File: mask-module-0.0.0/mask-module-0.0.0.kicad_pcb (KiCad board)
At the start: 2 copper layers, 17.8 x 33 mm, 27 parts, among them J1 Conn_01x02, J2 USB_C_Receptacle_USB2.0, J3 Conn_ARM_JTAG_SWD_10, J4 Conn_01x02, J5 Conn_01x13, J6 Conn_01x13, U1 BQ24075RGT, U3 MCP1703Ax-330xxTT, U4 BMD-380, Y1 FC-135 32.768KA-A5

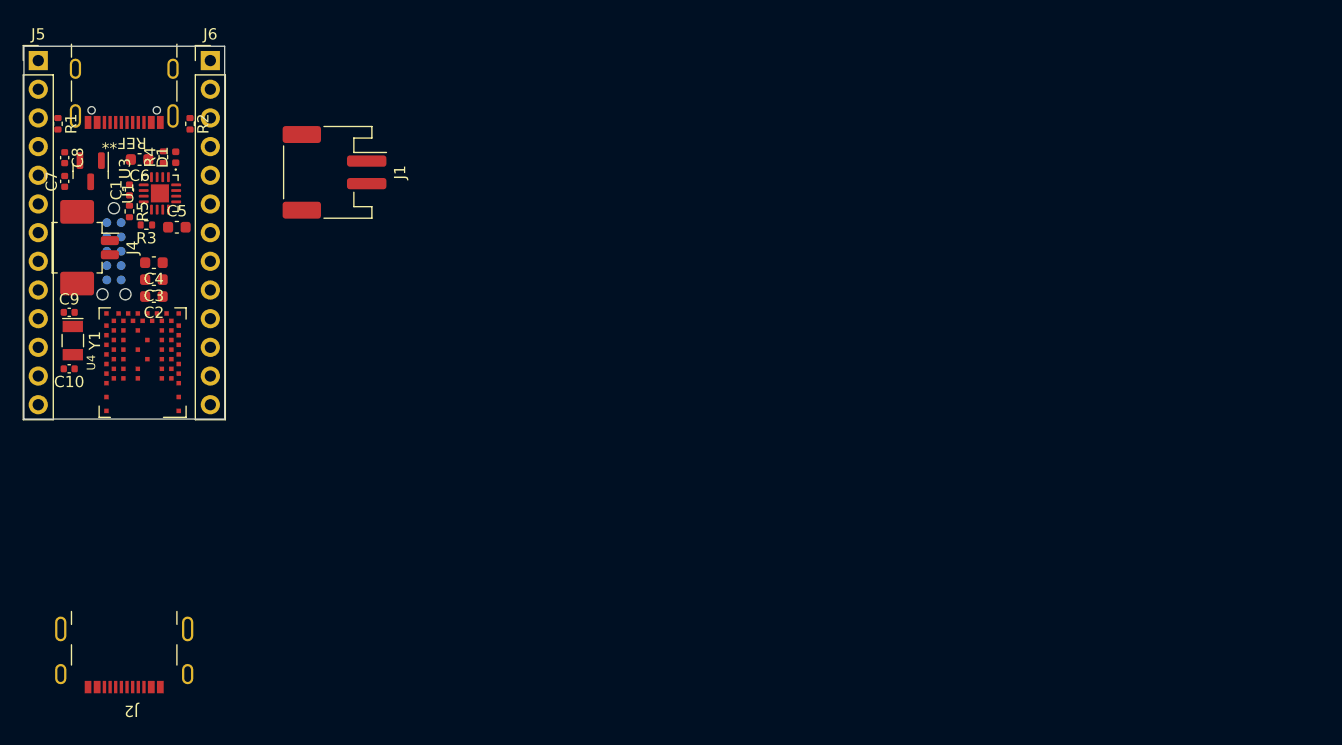
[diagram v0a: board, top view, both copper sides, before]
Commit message: module-0.0.0: finish pcb
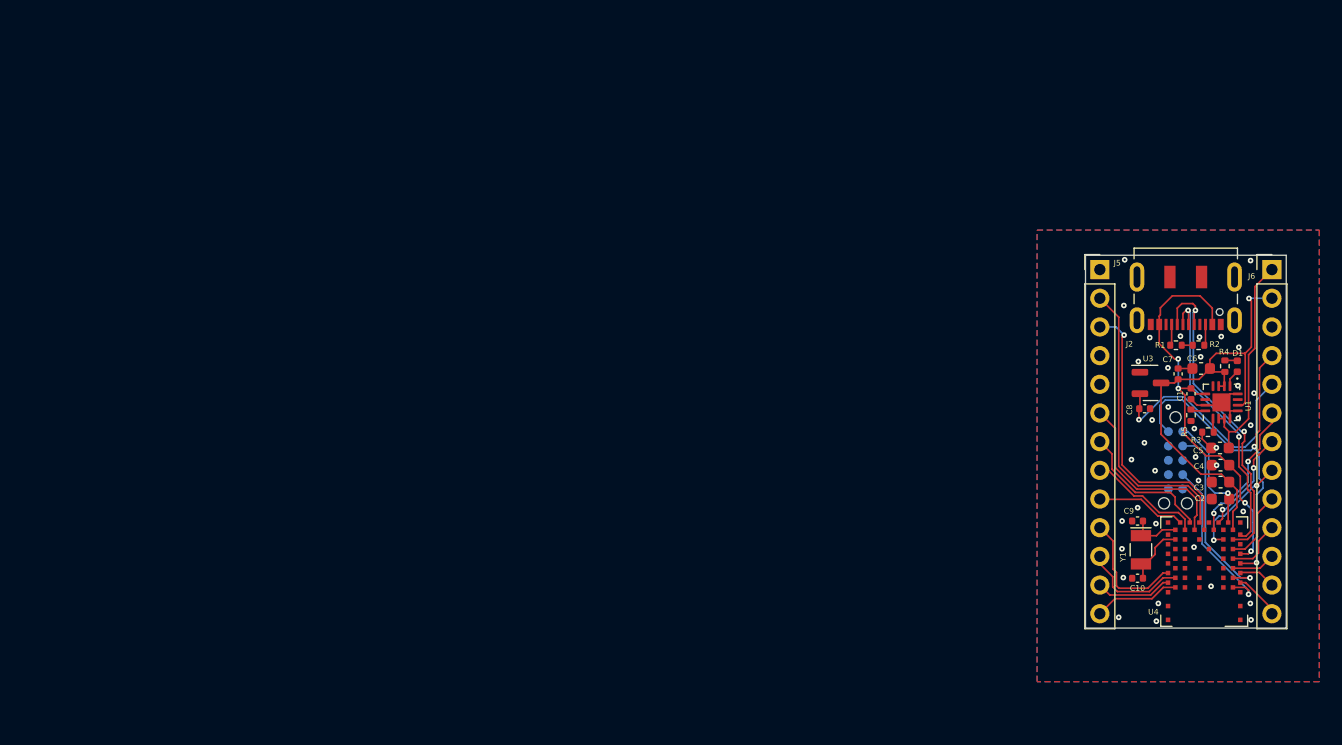
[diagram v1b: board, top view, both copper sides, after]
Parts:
- removed J1: Conn_01x02, Connector_JST:JST_PH_S2B-PH-SM4-TB_1x02-1MP_P2.00mm_Horizontal
- removed J4: Conn_01x02, Connector_Molex:Molex_PicoBlade_53261-0271_1x02-1MP_P1.25mm_Horizontal
- removed REF**: USB_C_Receptacle_GCT_USB4105-xx-A_16P_TopMnt_Horizontal, Connector_USB:USB_C_Receptacle_GCT_USB4105-xx-A_16P_TopMnt_Horizontal
- J2: footprint mask:USB_C_Receptacle_GCT_USB4520-xx-x-A_16P_Horizontal -> Connector_USB:USB_C_Receptacle_JAE_DX07S016JA1R1500
- moved R1 100.9 mm to (136.3, 88.7), turned to 0 degrees
- moved C7 100.1 mm to (136.5, 91.3)
- moved J2 99.3 mm to (137.2, 83.8)
- moved C8 98.2 mm to (133.6, 94.3), turned to 0 degrees
- moved C10 96.4 mm to (132.9, 109.4)
- moved C9 96.4 mm to (132.9, 104.3)
- moved Y1 96.4 mm to (133.2, 106.8)
- moved C2 96.2 mm to (140.3, 102.3)
- moved C3 96.2 mm to (140.3, 100.8)
- moved C4 96.2 mm to (140.3, 99.3)
- moved C6 95.8 mm to (138.6, 90.8)
- moved J5 95.8 mm to (129.6, 82.0)
- moved R4 95.8 mm to (140.7, 90.6)
- moved D1 95.8 mm to (141.8, 90.6)
- moved J3 95.8 mm to (136.3, 98.9)
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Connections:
- J5 pad 10: P1.00 -> P1.10
- J5 pad 11: P0.11 -> P1.06
- J5 pad 12: P1.04 -> P0.10
- J5 pad 13: P1.06 -> P0.09
- J5 pad 6: P0.17 -> P0.05
- J5 pad 7: P0.20 -> P0.27
- J5 pad 8: P0.22 -> P0.26
- J5 pad 9: P0.24 -> P0.04
- J6 pad 10: P1.13 -> P0.17
- J6 pad 11: P1.11 -> P0.21
- J6 pad 12: P0.10 -> P0.19
- J6 pad 13: P0.09 -> P0.22
- J6 pad 6: P0.31 -> P0.07
- J6 pad 7: P0.29 -> P0.12
- J6 pad 8: P0.02 -> P0.15
- J6 pad 9: P1.15 -> P0.14
- U4 pad 10: unconnected-(U4-P0.21-Pad10) -> P0.21
- U4 pad 16: unconnected-(U4-P0.14-Pad16) -> P0.14
- U4 pad 20: unconnected-(U4-P0.15-Pad20) -> P0.15
- U4 pad 26: unconnected-(U4-P0.12/TRACEDATA[1]-Pad26) -> P0.12
- U4 pad 27: unconnected-(U4-P0.07/TRACECLK-Pad27) -> P0.07
- U4 pad 31: unconnected-(U4-P0.05/AIN3-Pad31) -> P0.05
- U4 pad 32: unconnected-(U4-P0.27-Pad32) -> P0.27
- U4 pad 33: unconnected-(U4-P0.26-Pad33) -> P0.26
- U4 pad 34: unconnected-(U4-P0.04/AIN2-Pad34) -> P0.04
- U4 pad 49: unconnected-(U4-P1.10-Pad49) -> P1.10
- U4 pad 8: unconnected-(U4-P0.25-Pad8) -> P0.25
- U4 pad 9: unconnected-(U4-P0.19-Pad9) -> P0.19
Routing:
- net +5V: track 0.00 -> 41.6 mm, vias 0 -> 1
- net VBUS: track 0.00 -> 36.6 mm, vias 0 -> 4
- net RESET: track 0.00 -> 34.1 mm, vias 0 -> 2
- net D-: track 0.00 -> 29.4 mm, vias 0 -> 2
- net P0.06_TXD: track 0.00 -> 26.2 mm
- net D+: track 0.00 -> 25.8 mm, vias 0 -> 2
- net P0.08_RXD: track 0.00 -> 25.4 mm, vias 0 -> 1
- net +3V3: track 0.00 -> 21.0 mm, vias 0 -> 1
- net VBAT: track 0.00 -> 19.6 mm
- net SWDIO: track 0.00 -> 16.8 mm, vias 0 -> 1
- net P0.05: track 0.00 -> 16.6 mm
- net SWCLK: track 0.00 -> 14.9 mm, vias 0 -> 1
- net P0.07: track 0.00 -> 12.8 mm, vias 0 -> 2
- net P0.27: track 0.00 -> 12.3 mm
- net GND: track 0.00 -> 11.2 mm, vias 0 -> 38
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- added copper zone on B.Cu, net GND
- added copper zone on F.Cu, net GND
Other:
- board text removed: "InsightSIP ISP1807-LR-RS"
- board text removed: "ublox BMD-380"
